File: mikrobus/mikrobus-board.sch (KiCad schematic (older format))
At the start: 7 parts, among them J1 Conn_01x04, P3 microBus_1, P4 microBus_2, P5 microBus_1, P6 microBus_2

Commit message: update connector
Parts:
- removed J1: Conn_01x04, Pin_Headers:Pin_Header_Straight_1x04_Pitch2.54mm, symbol Conn_01x04
- added J1: Conn_01x06, Pin_Headers:Pin_Header_Straight_1x06_Pitch2.54mm, symbol Conn_01x06
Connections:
- wire segments 72 -> 74
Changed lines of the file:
@@
 $EndComp
 $Comp
-L +3.3V #PWR01
+L +3.3V #PWR9
 U 1 1 5A7F089C
 P 8200 6300
-F 0 "#PWR01" H 8200 6150 50  0001 C CNN
+F 0 "#PWR9" H 8200 6150 50  0001 C CNN
 F 1 "+3.3V" H 8200 6440 50  0000 C CNN
 F 2 "" H 8200 6300 50  0001 C CNN
@@
 TX_1
 $Comp
-L GND #PWR02
+L GND #PWR3
 U 1 1 5732FDAE
 P 4750 8000
-F 0 "#PWR02" H 4750 7750 50  0001 C CNN
+F 0 "#PWR3" H 4750 7750 50  0001 C CNN
 F 1 "GND" H 4750 7850 50  0000 C CNN
 F 2 "" H 4750 8000 50  0000 C CNN
@@
 RST_1
 $Comp
-L +3.3V #PWR03
+L +3.3V #PWR1
 U 1 1 5ABB8932
 P 3350 7800
-F 0 "#PWR03" H 3350 7650 50  0001 C CNN
+F 0 "#PWR1" H 3350 7650 50  0001 C CNN
 F 1 "+3.3V" H 3350 7940 50  0000 C CNN
 F 2 "" H 3350 7800 50  0001 C CNN
@@
 TX_2
 $Comp
-L GND #PWR04
+L GND #PWR6
 U 1 1 5ABB8B45
 P 6100 8000
-F 0 "#PWR04" H 6100 7750 50  0001 C CNN
+F 0 "#PWR6" H 6100 7750 50  0001 C CNN
 F 1 "GND" H 6100 7850 50  0000 C CNN
 F 2 "" H 6100 8000 50  0000 C CNN
@@
 $EndComp
 $Comp
-L GND #PWR05
+L GND #PWR7
 U 1 1 5ABB8B4B
 P 7200 8000
-F 0 "#PWR05" H 7200 7750 50  0001 C CNN
+F 0 "#PWR7" H 7200 7750 50  0001 C CNN
 F 1 "GND" H 7200 7850 50  0000 C CNN
 F 2 "" H 7200 8000 50  0000 C CNN
@@
 RST_2
 NoConn ~ 7550 5300
-$Comp
-L Conn_01x04 J1
-U 1 1 5ABB9346
-P 9650 7250
-F 0 "J1" H 9650 7450 50  0000 C CNN
-F 1 "Conn_01x04" H 9650 6950 50  0000 C CNN
-F 2 "Pin_Headers:Pin_Header_Straight_1x04_Pitch2.54mm" H 9650 7250 50  0001 C CNN
-F 3 "" H 9650 7250 50  0001 C CNN
-	1    9650 7250
-	1    0    0    -1
-$EndComp
 Text Label 8950 7150 0    60   ~ 0
 EXT_1
@@
 EXT_4
 $Comp
-L GND #PWR06
+L GND #PWR5
 U 1 1 5ABB9FEC
 P 5950 6450
-F 0 "#PWR06" H 5950 6200 50  0001 C CNN
+F 0 "#PWR5" H 5950 6200 50  0001 C CNN
 F 1 "GND" H 5950 6300 50  0000 C CNN
 F 2 "" H 5950 6450 50  0001 C CNN
@@
 $EndComp
 $Comp
-L +3.3V #PWR07
+L +3.3V #PWR4
 U 1 1 5ABBA05D
 P 5850 7800
-F 0 "#PWR07" H 5850 7650 50  0001 C CNN
+F 0 "#PWR4" H 5850 7650 50  0001 C CNN
 F 1 "+3.3V" H 5850 7940 50  0000 C CNN
 F 2 "" H 5850 7800 50  0001 C CNN
@@
 	5850 7800 6200 7800
 $Comp
-L GND #PWR08
+L GND #PWR2
 U 1 1 5ABBA17A
 P 3650 7900
-F 0 "#PWR08" H 3650 7650 50  0001 C CNN
+F 0 "#PWR2" H 3650 7650 50  0001 C CNN
 F 1 "GND" H 3650 7750 50  0000 C CNN
 F 2 "" H 3650 7900 50  0001 C CNN
@@
 $EndComp
 $Comp
-L GND #PWR09
+L GND #PWR8
 U 1 1 5ABBA41C
 P 8150 6100
-F 0 "#PWR09" H 8150 5850 50  0001 C CNN
+F 0 "#PWR8" H 8150 5850 50  0001 C CNN
 F 1 "GND" H 8150 5950 50  0000 C CNN
 F 2 "" H 8150 6100 50  0001 C CNN
@@
 Wire Wire Line
 	7550 6100 8150 6100
+$Comp
+L Conn_01x06 J1
+U 1 1 5ABB93C6
+P 9650 7350
+F 0 "J1" H 9650 7650 50  0000 C CNN
+F 1 "Conn_01x06" H 9650 6950 50  0000 C CNN
+F 2 "Pin_Headers:Pin_Header_Straight_1x06_Pitch2.54mm" H 9650 7350 50  0001 C CNN
+F 3 "" H 9650 7350 50  0001 C CNN
+	1    9650 7350
+	1    0    0    -1
+$EndComp
+$Comp
+L +3.3V #PWR10
+U 1 1 5ABB93FE
+P 9150 7550
+F 0 "#PWR10" H 9150 7400 50  0001 C CNN
+F 1 "+3.3V" H 9150 7690 50  0000 C CNN
+F 2 "" H 9150 7550 50  0001 C CNN
+F 3 "" H 9150 7550 50  0001 C CNN
+	1    9150 7550
+	0    -1   -1   0
+$EndComp
+$Comp
+L GND #PWR11
+U 1 1 5ABB9420
+P 9150 7650
+F 0 "#PWR11" H 9150 7400 50  0001 C CNN
+F 1 "GND" H 9150 7500 50  0000 C CNN
+F 2 "" H 9150 7650 50  0001 C CNN
+F 3 "" H 9150 7650 50  0001 C CNN
+	1    9150 7650
+	0    1    1    0
+$EndComp
+Wire Wire Line
+	9150 7650 9450 7650
+Wire Wire Line
+	9150 7550 9450 7550
 $EndSCHEMATC

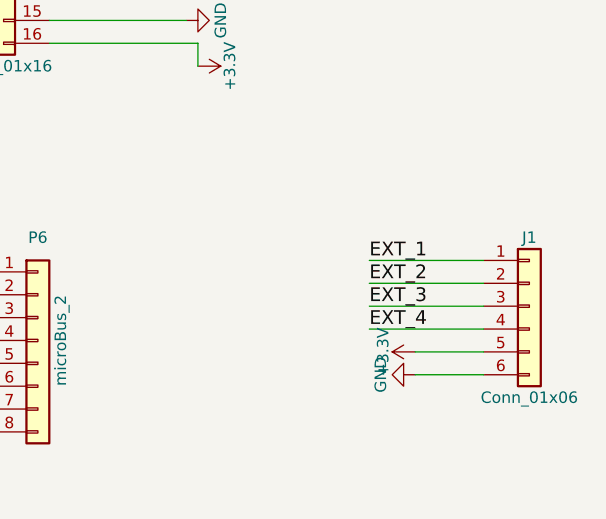
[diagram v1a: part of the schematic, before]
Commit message: Finished routing
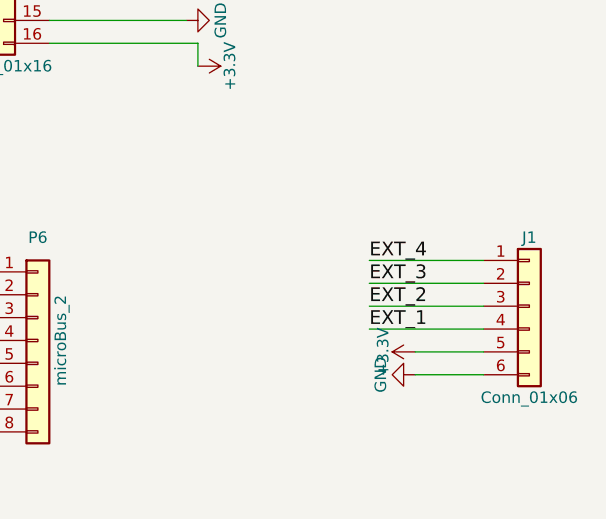
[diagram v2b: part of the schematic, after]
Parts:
- P3, P4, P5, P6: footprint Pin_Headers:Pin_Header_Straight_1x08_Pitch2.54mm -> Socket_Strips:Socket_Strip_Straight_1x08_Pitch2.54mm
- UPDUINO2_DOWN1: footprint Pin_Headers:Pin_Header_Straight_1x16_Pitch2.54mm -> Socket_Strips:Socket_Strip_Straight_1x16_Pitch2.54mm
- UPDUINO2_UP1: footprint Pin_Headers:Pin_Header_Straight_1x18_Pitch2.54mm -> Socket_Strips:Socket_Strip_Straight_1x18_Pitch2.54mm
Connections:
- net EXT_1: now also J1.4 (Pin_4); no longer J1.1 (Pin_1)
- net EXT_2: now also J1.3 (Pin_3); no longer J1.2 (Pin_2)
- net EXT_3: now also J1.2 (Pin_2); no longer J1.3 (Pin_3)
- net EXT_4: now also J1.1 (Pin_1); no longer J1.4 (Pin_4)
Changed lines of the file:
@@
 EESchema Schematic File Version 2
-LIBS:mikrobus-board-rescue
 LIBS:power
 LIBS:device
@@
 F 0 "UPDUINO2_UP1" H 6700 6400 50  0000 C CNN
 F 1 "Conn_01x18" H 6700 4500 50  0000 C CNN
-F 2 "Pin_Headers:Pin_Header_Straight_1x18_Pitch2.54mm" H 6700 5500 50  0001 C CNN
+F 2 "Socket_Strips:Socket_Strip_Straight_1x18_Pitch2.54mm" H 6700 5500 50  0001 C CNN
 F 3 "" H 6700 5500 50  0001 C CNN
 	1    6700 5500
@@
 F 0 "UPDUINO2_DOWN1" H 7350 6200 50  0000 C CNN
 F 1 "Conn_01x16" H 7350 4500 50  0000 C CNN
-F 2 "Pin_Headers:Pin_Header_Straight_1x16_Pitch2.54mm" H 7350 5400 50  0001 C CNN
+F 2 "Socket_Strips:Socket_Strip_Straight_1x16_Pitch2.54mm" H 7350 5400 50  0001 C CNN
 F 3 "" H 7350 5400 50  0001 C CNN
 	1    7350 5400
@@
 F 0 "P3" H 3950 7950 50  0000 C CNN
 F 1 "microBus_1" V 4050 7500 50  0000 C CNN
-F 2 "Pin_Headers:Pin_Header_Straight_1x08_Pitch2.54mm" H 3950 7500 50  0001 C CNN
+F 2 "Socket_Strips:Socket_Strip_Straight_1x08_Pitch2.54mm" H 3950 7500 50  0001 C CNN
 F 3 "" H 3950 7500 50  0000 C CNN
 	1    3950 7500
@@
 F 0 "P4" H 5050 7950 50  0000 C CNN
 F 1 "microBus_2" V 5150 7500 50  0000 C CNN
-F 2 "Pin_Headers:Pin_Header_Straight_1x08_Pitch2.54mm" H 5050 7500 50  0001 C CNN
+F 2 "Socket_Strips:Socket_Strip_Straight_1x08_Pitch2.54mm" H 5050 7500 50  0001 C CNN
 F 3 "" H 5050 7500 50  0000 C CNN
 	1    5050 7500
@@
 F 0 "P5" H 6400 7950 50  0000 C CNN
 F 1 "microBus_1" V 6500 7500 50  0000 C CNN
-F 2 "Pin_Headers:Pin_Header_Straight_1x08_Pitch2.54mm" H 6400 7500 50  0001 C CNN
+F 2 "Socket_Strips:Socket_Strip_Straight_1x08_Pitch2.54mm" H 6400 7500 50  0001 C CNN
 F 3 "" H 6400 7500 50  0000 C CNN
 	1    6400 7500
@@
 F 0 "P6" H 7500 7950 50  0000 C CNN
 F 1 "microBus_2" V 7600 7500 50  0000 C CNN
-F 2 "Pin_Headers:Pin_Header_Straight_1x08_Pitch2.54mm" H 7500 7500 50  0001 C CNN
+F 2 "Socket_Strips:Socket_Strip_Straight_1x08_Pitch2.54mm" H 7500 7500 50  0001 C CNN
 F 3 "" H 7500 7500 50  0000 C CNN
 	1    7500 7500
@@
 NoConn ~ 7550 5300
 Text Label 8950 7150 0    60   ~ 0
+EXT_4
+Text Label 8950 7250 0    60   ~ 0
+EXT_3
+Text Label 8950 7350 0    60   ~ 0
+EXT_2
+Text Label 8950 7450 0    60   ~ 0
 EXT_1
-Text Label 8950 7250 0    60   ~ 0
-EXT_2
-Text Label 8950 7350 0    60   ~ 0
-EXT_3
-Text Label 8950 7450 0    60   ~ 0
-EXT_4
 $Comp
 L GND #PWR5
